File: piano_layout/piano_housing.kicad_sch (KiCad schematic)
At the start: 24 parts, among them SW1 C, SW10 A, SW11 A#, SW12 B, SW13 C O, SW14 C# O, SW15 D O, SW16 D# O, SW17 E O, SW18 F O, SW19 F# O, SW2 C#, SW20 G O, SW21 G# O, SW22 A O, SW23 A# O, SW24 B O, SW3 D, SW4 D#, SW5 E, SW6 F, SW7 F#, SW8 G, SW9 G#

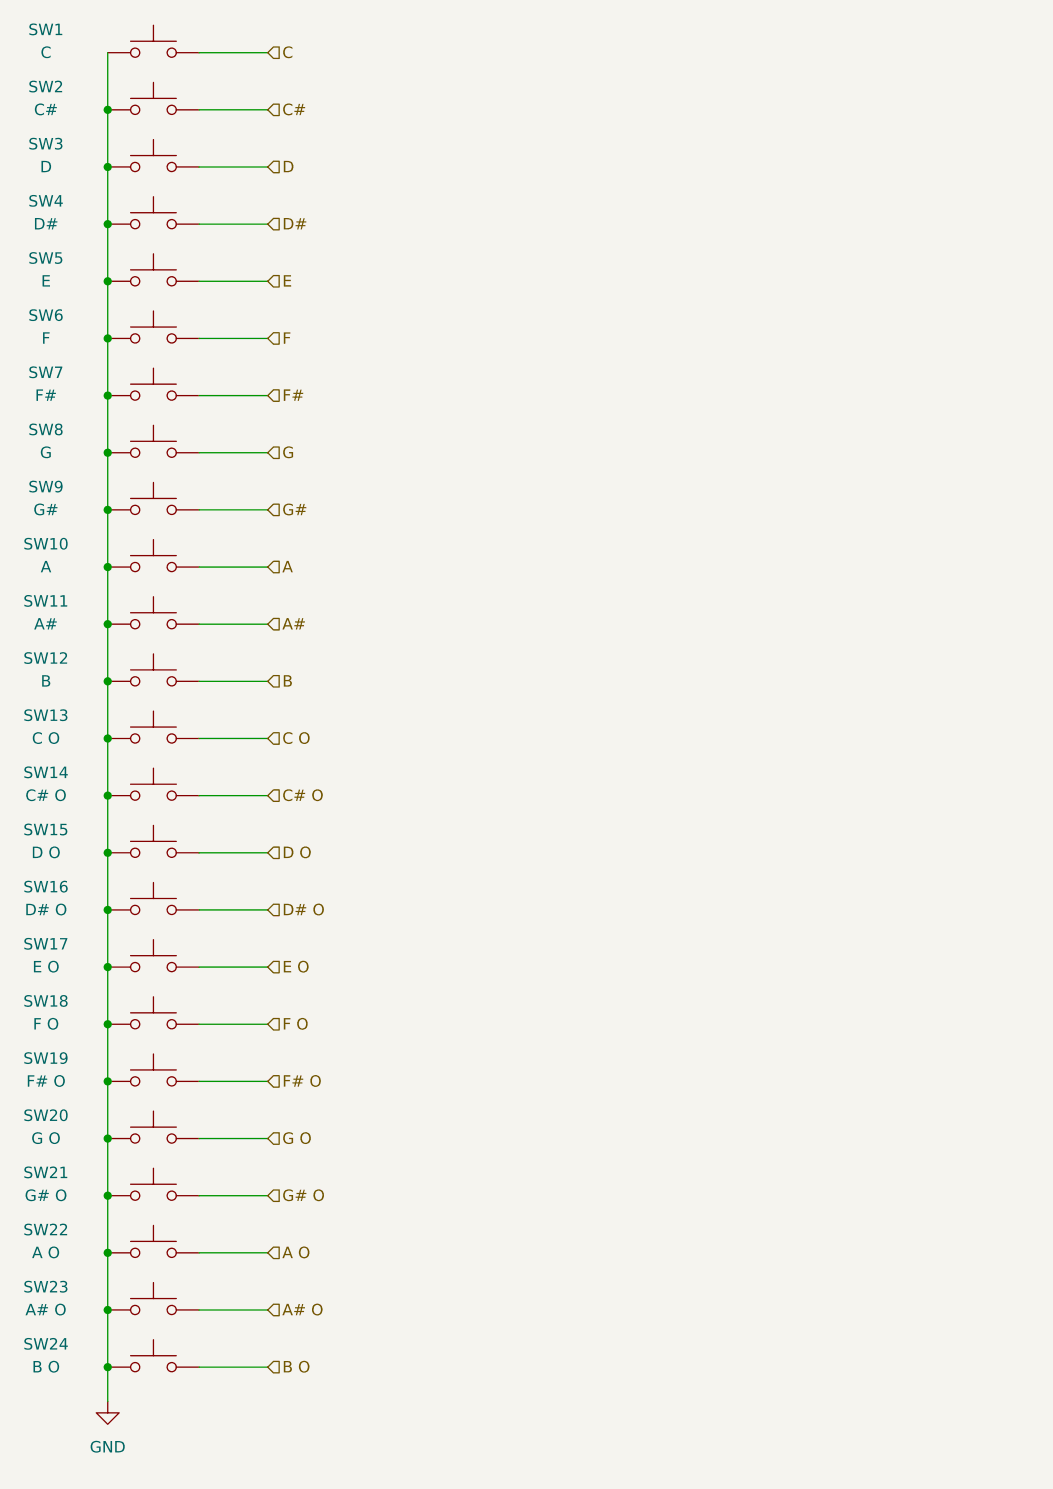
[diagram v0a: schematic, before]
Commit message: updated readme
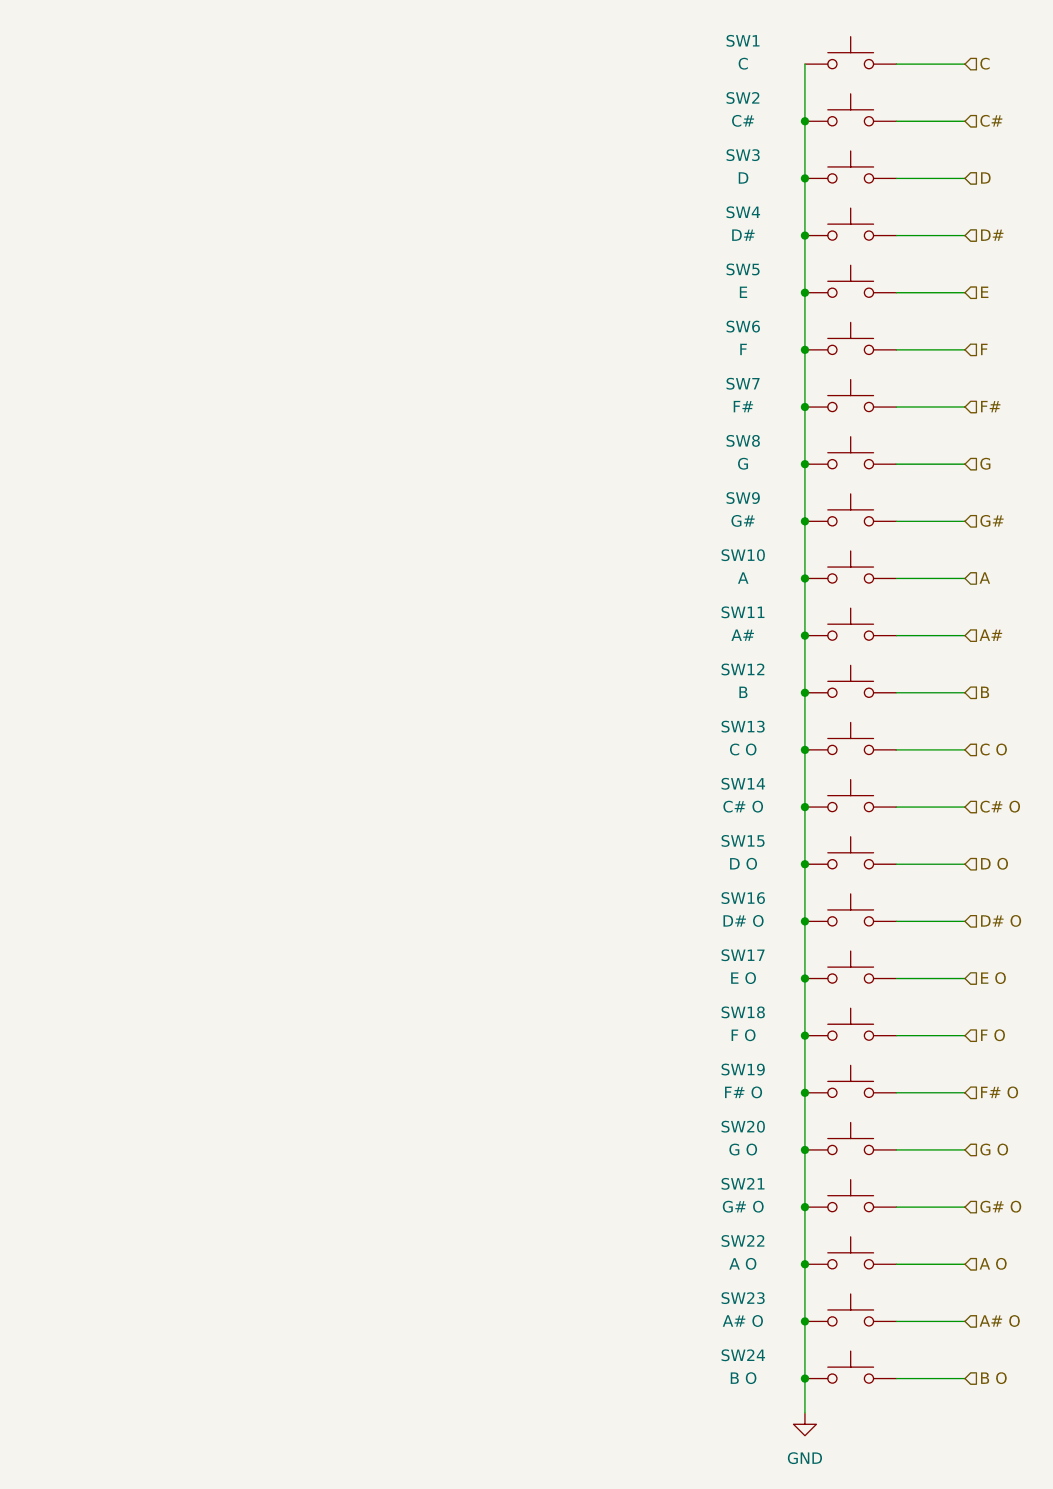
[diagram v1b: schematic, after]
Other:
- title: (none) -> Piano Button Housing
- moved on the sheet: SW1, SW10, SW11, SW12, SW13, SW14, SW15, SW16, SW17, SW18, SW19, SW2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
